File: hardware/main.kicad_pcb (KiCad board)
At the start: 2 copper layers, 98 x 68.3 mm, 19 parts, among them J3 Conn_01x01_Pin, J4 Conn_01x01_Pin, J5 Conn_01x01_Pin, J6 Conn_01x01_Pin, K2 ADW11

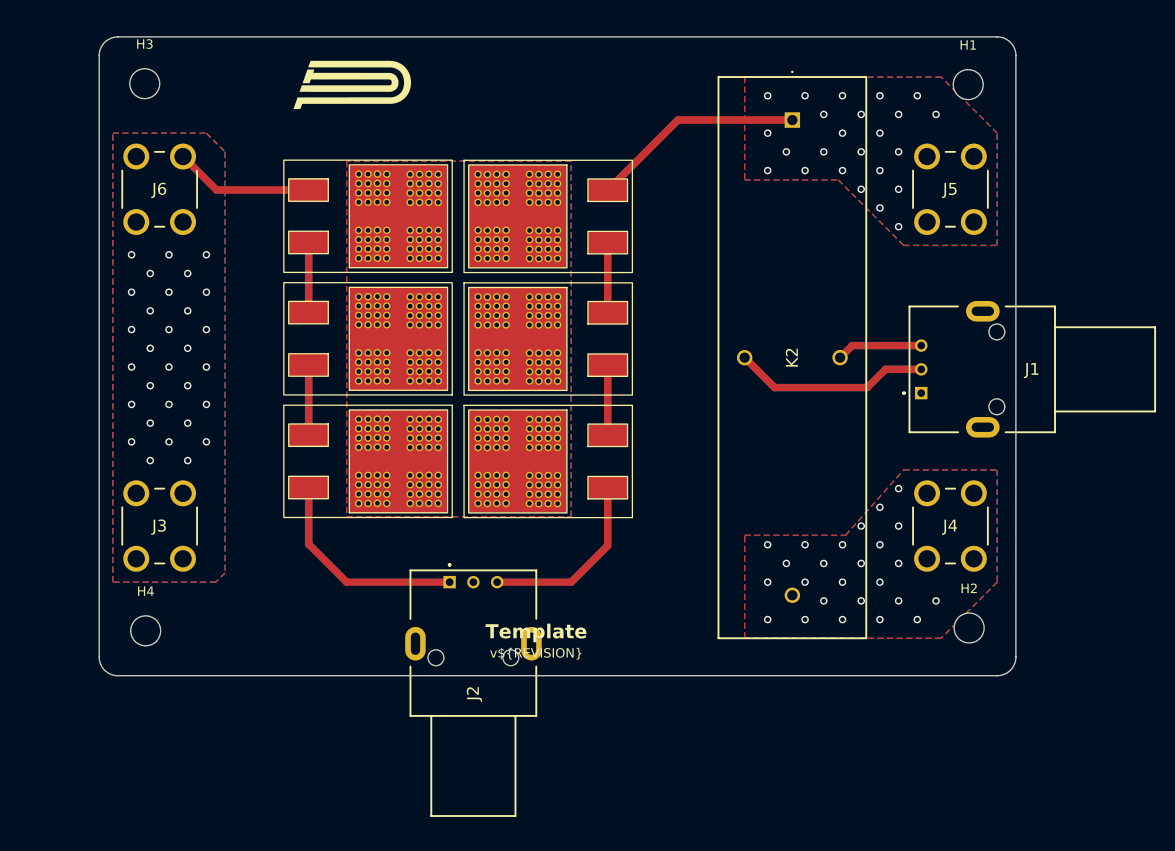
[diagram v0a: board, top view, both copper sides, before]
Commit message: Fabrication Toolkit files added
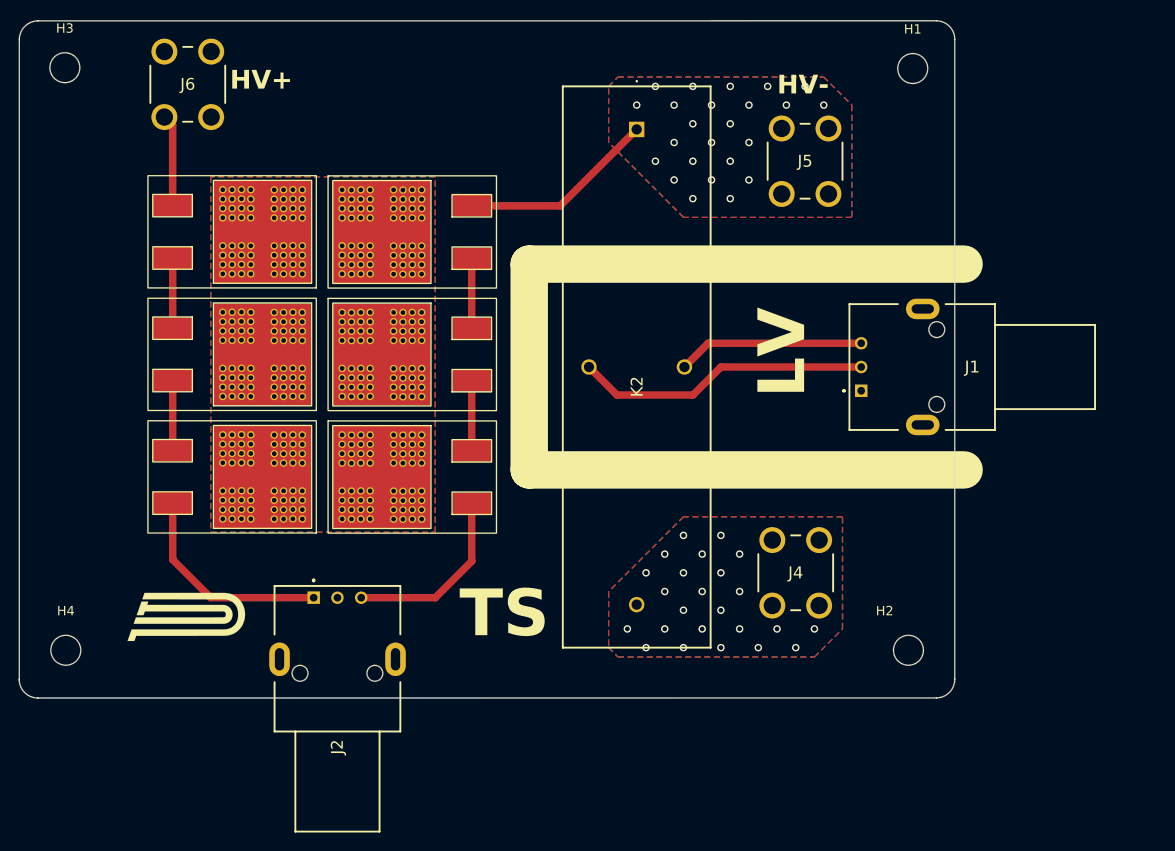
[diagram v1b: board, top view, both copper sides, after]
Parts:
- removed J3: Conn_01x01_Pin, 7696:7696
- moved G*** 59.6 mm to (124.5, 109.6)
- moved J4 17.3 mm to (187.5, 108.5)
- moved K2 16.7 mm to (173.0, 57.6)
- moved J5 15.8 mm to (188.5, 64.5)
- moved G*** 14.6 mm to (150.0, 53.0)
- moved J2 14.6 mm to (138.5, 107.7)
- moved PWR263S-35-5001F2 14.6 mm to (127.7, 81.6)
- moved PWR263S-35-5001F3 14.6 mm to (127.7, 94.7)
- moved PWR263S-35-5001F4 14.6 mm to (151.0, 94.8)
- moved PWR263S-35-5001F5 14.6 mm to (151.0, 81.7)
- moved PWR263S-35-5001F1 14.6 mm to (127.7, 68.5)
- moved PWR263S-35-5001F6 14.6 mm to (151.0, 68.6)
- moved J6 11.6 mm to (127.5, 49.3)
- moved H4 8.79 mm to (112.0, 113.3)
- moved H3 8.71 mm to (111.9, 51.0)
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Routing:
- net GND: track 9.31 -> 20.0 mm
- net SD+: track 21.0 -> 31.6 mm
- net HV+: track 14.9 -> 9.82 mm, vias 30 -> 0
- net HV-: track 22.9 -> 21.0 mm
- net Net-(J4-Pin_1): vias 25 -> 24
- removed copper zone on B.Cu, net HV+
- removed copper zone on F.Cu, net HV+
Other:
- board size 98 x 68.3 mm -> 100 x 72.4 mm
- board text added: "HV+"
- board text added: "HV-"
- board text added: "LV"
- board text added: "TS"
- board text removed: "Template"
- board text removed: "v${REVISION}"
